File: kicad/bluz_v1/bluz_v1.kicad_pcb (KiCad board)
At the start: 2 copper layers, 24.9 x 14.9 mm, 70 parts, among them J1 USB_B_Micro, J10 Conn, J11 Conn, J12 BTAnt, J2 Conn, J3 Conn, J4 Conn, J5 Conn, J6 Conn, J7 Conn, J8 Conn, J9 Conn, M1 VibroMotor, Q1 RUM002N05, Q2 RUM002N05, SW1 SW_DPDT_x2, U1 MCP73831, U2 MCP1700, U3 TLV3201AIDCK, U4 AP3015KTR, Y1 NX1612SA-32MHz, Y2 NX1610-32.768

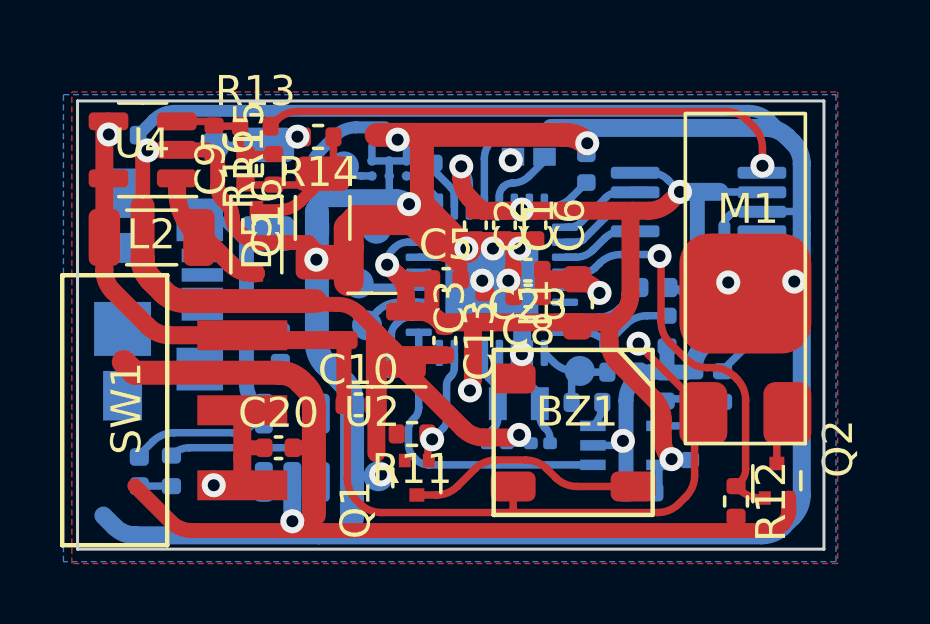
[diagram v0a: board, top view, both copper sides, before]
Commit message: изменено:      kicad/bluz_v1/bluz_v1.kicad_pcb 	изменено:      kicad/bluz_v1/bluz_v1.kicad_sch 	изменено:      stm32cubeide/BluZ_v1/.cproject 	изменено:      stm32cubeide/BluZ_v1/.mxproject 	изменено:      stm32cubeide/BluZ_v1/.settings/language.settings.xml 	изменено:      stm32cubeide/BluZ_v1/BluZ_v1.ioc 	изменено:      stm32cubeide/BluZ_v1/Core/Inc/app_conf.h 	изменено:      stm32cubeide/BluZ_v1/Core/Inc/main.h 	изменено:      stm32cubeide/BluZ_v1/Core/Inc/stm32wbaxx_it.h 	изменено:      stm32cubeide/BluZ_v1/Core/Src/app_entry.c 	изменено:      stm32cubeide/BluZ_v1/Core/Src/main.c 	изменено:      stm32cubeide/BluZ_v1/Core/Src/stm32wbaxx_hal_msp.c 	изменено:      stm32cubeide/BluZ_v1/Core/Src/stm32wbaxx_it.c
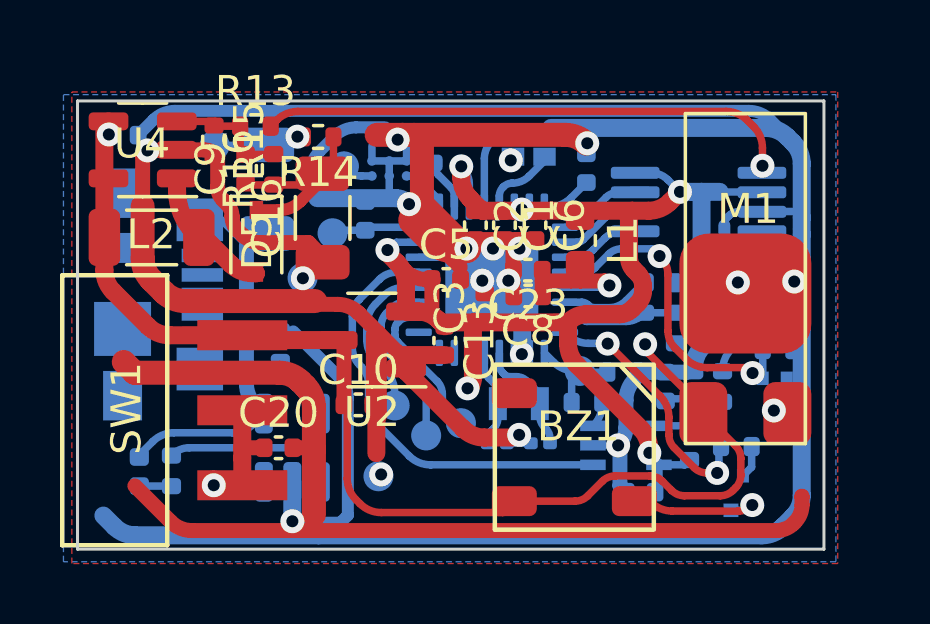
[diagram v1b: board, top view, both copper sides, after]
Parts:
- D4: value LTC1661CMS8 -> LTC1662CMS8
- L1: value 47uH -> 10uH
- Q1, Q2, R11, R12: moved to B.Cu
- moved R11 10.8 mm to (83.7, 48.6), turned to 0 degrees
- moved Q1 10.5 mm to (83.5, 50.2)
- moved R12 5.25 mm to (85.0, 45.4), turned to 0 degrees
- moved J9 4.24 mm to (72.3, 47.3)
- moved J4 4.17 mm to (73.3, 48.3)
- moved J5 3.06 mm to (74.5, 47.9)
- moved Q2 2.84 mm to (84.9, 46.9), turned to -90 degrees
- moved L1 2.08 mm to (78.5, 41.8), turned to -90 degrees
- moved J2 1.47 mm to (70.2, 41.5)
- moved C18 1.09 mm to (71.3, 40.9), turned to -90 degrees
- moved R1 0.90 mm to (80.6, 44.7), turned to 90 degrees
- moved J10 0.77 mm to (69.2, 43.0)
- moved BZ1 0.49 mm to (78.3, 48.6)
- moved R2 0.30 mm to (81.6, 44.7)
- moved C11 0.26 mm to (83.1, 42.7)
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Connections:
- D1 pad 15: Sound -> unconnected-(D1-Pad15)
- D1 pad 17: Sync -> unconnected-(D1-Pad17)
- D1 pad 21: unconnected-(D1-Pad21) -> Sync
- D1 pad 6: unconnected-(D1-Pad6) -> LED
- D1 pad 7: LED -> batLev
- D1 pad 8: batLev -> Sound
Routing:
- net GND: track 208.7 -> 203.0 mm
- net Sound: track 4.47 -> 8.57 mm, vias 1 -> 2
- net Sync: track 10.5 -> 14.6 mm
- net /swd: track 1.93 -> 5.88 mm
- net /TxD: track 1.91 -> 5.37 mm
- net Vibro: track 13.9 -> 10.6 mm, vias 1 -> 2
- net Net-(BZ1-Pad2): track 7.86 -> 4.86 mm, vias 0 -> 1
- net /swc: track 2.18 -> 4.97 mm
- net Net-(M1-Pad1): track 1.81 -> 0.00 mm, vias 0 -> 1
- net +BATT: track 37.0 -> 38.6 mm
- net Net-(C23-Pad1): track 4.22 -> 5.44 mm

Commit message: изменено:      kicad/bluz_v1/bluz_v1.kicad_pcb 	изменено:      kicad/bluz_v1/bluz_v1.kicad_prl 	изменено:      kicad/bluz_v1/fp-info-cache
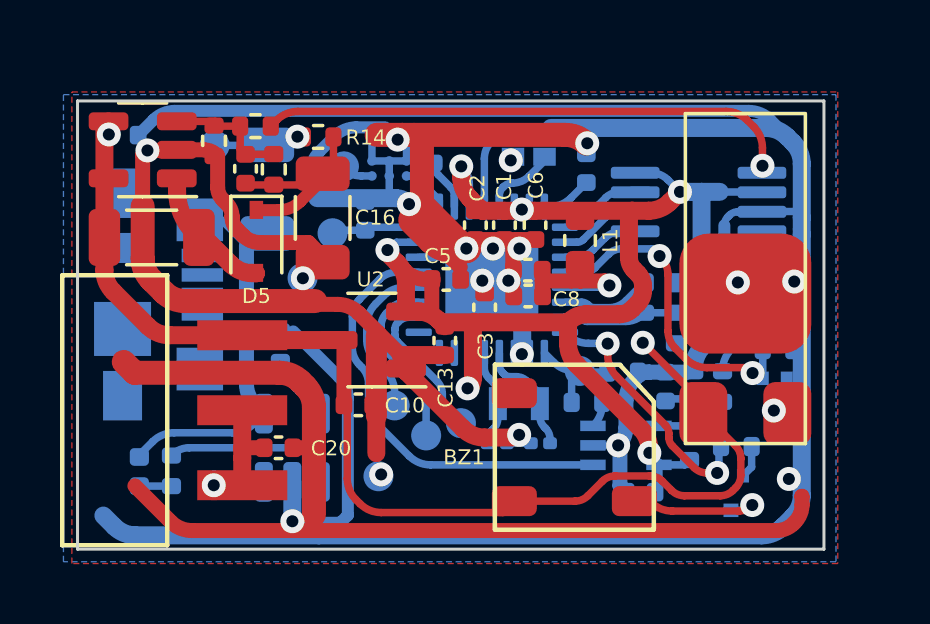
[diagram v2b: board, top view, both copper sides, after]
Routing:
- net GND: vias 18 -> 19
